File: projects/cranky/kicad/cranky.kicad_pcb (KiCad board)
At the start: 2 copper layers, 50 x 50 mm, 51 parts, among them CON1 USB-MINI-B, P1 ISP, P2 CONN_01X04, P3 CONN_01X04, P4 CONN_01X04, P5 CONN_01X04, Q1 2N7002P, Q2 2N7002P, Q3 ISL9V3040D3ST, Q4 ISL9V3040D3ST, Q5 VND5N07, Q6 VND5N07, SW1 SW_PUSH_SMALL, SW2 SW_PUSH_SMALL, U1 ATMEGA32U4-A, U2 LTV-826S, U3 LM7805CT, X1 16MHz

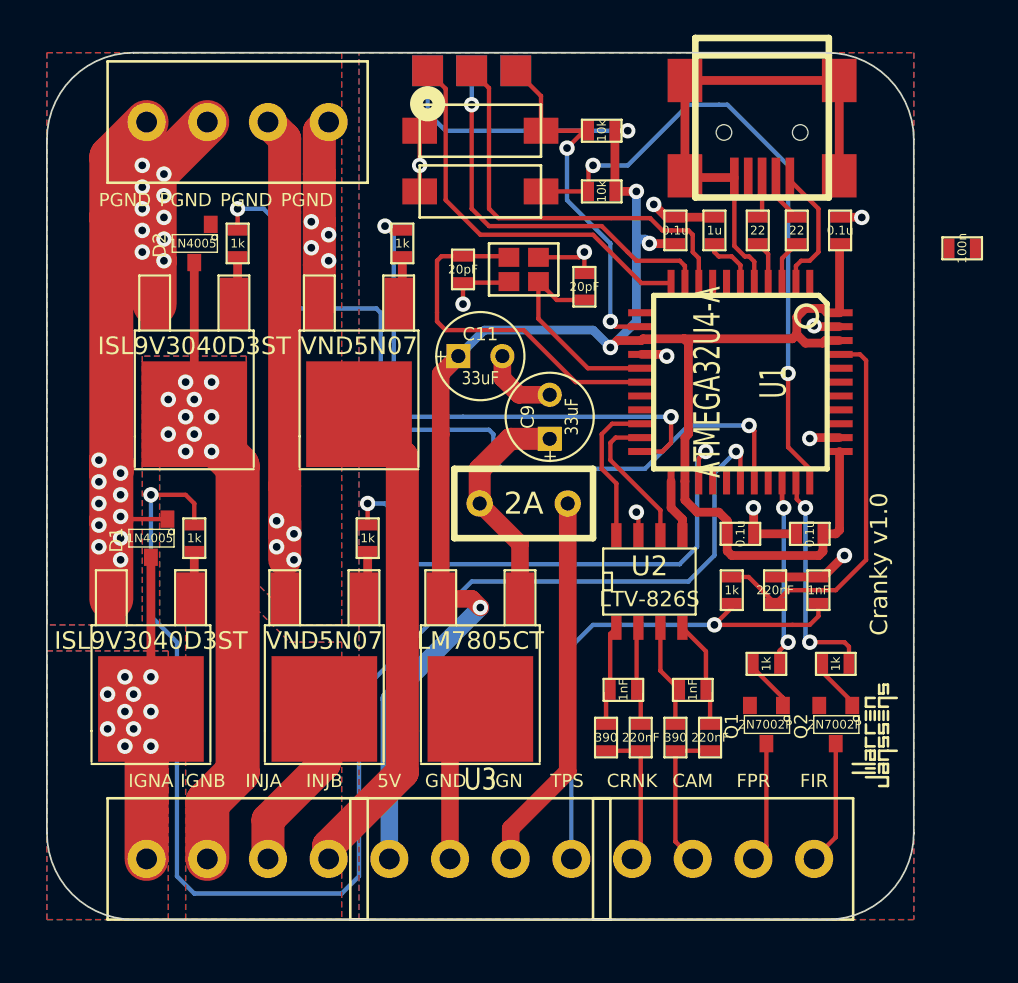
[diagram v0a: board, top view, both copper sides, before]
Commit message: routing new cranky board
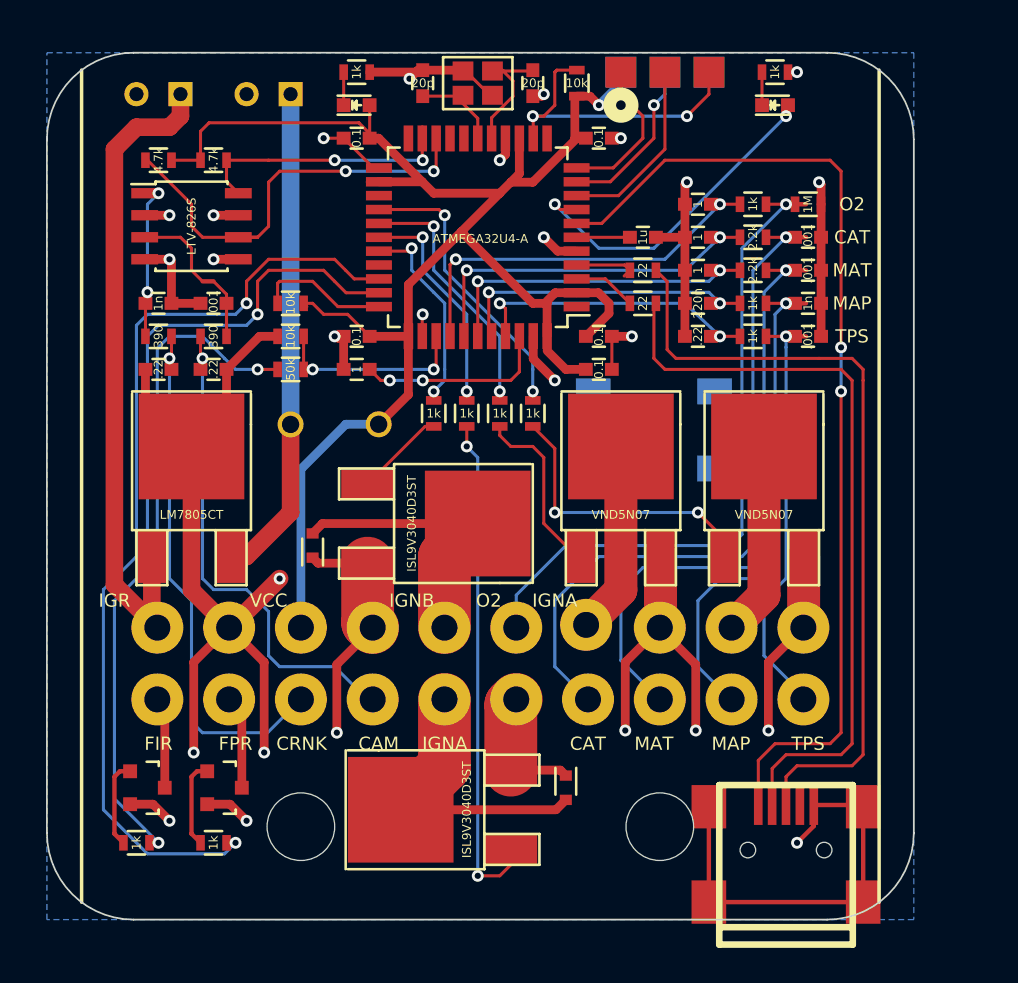
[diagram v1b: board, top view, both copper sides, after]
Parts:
- removed P3, P4, P5: CONN_01X04, SCREW_TERMINAL_4
- removed WJ10: VAL**, WJ10
- added C17: 0.1, Capacitors_SMD:C_0603, F.Cu at (76.8, 86.4)
- added C18: 1n, Capacitors_SMD:C_0603, F.Cu at (88.9, 84.5)
- added C19: .001, Capacitors_SMD:C_0603, F.Cu at (88.9, 80.6)
- added C20: .001, Capacitors_SMD:C_0603, F.Cu at (88.9, 82.5)
- added C21: 220n, Capacitors_SMD:C_0603, F.Cu at (82.5, 84.5)
- added C22: 1, Capacitors_SMD:C_0603, F.Cu at (82.5, 80.6)
- added C23: 1, Capacitors_SMD:C_0603, F.Cu at (82.5, 82.5)
- added C24: 1, Capacitors_SMD:C_0603, F.Cu at (82.5, 78.7)
- added D3: Led_Small, LEDs:LED-0603, F.Cu at (62.9, 73.0)
- added D4: Led_Small, LEDs:LED-0603, F.Cu at (87.0, 73.0)
- added R14: 4.7k, Resistors_SMD:R_0603, F.Cu at (54.6, 76.2)
- added R15: 4.7k, Resistors_SMD:R_0603, F.Cu at (51.4, 76.2)
- added R16: 1M, Resistors_SMD:R_0603, F.Cu at (88.9, 78.7)
- added R17: 50k, Resistors_SMD:R_0603, F.Cu at (59.1, 88.3)
- added R18: 1k, Resistors_SMD:R_0603, F.Cu at (85.7, 84.5)
- added R19: 2.2k, Resistors_SMD:R_0603, F.Cu at (85.7, 80.6)
- added R20: 2.2k, Resistors_SMD:R_0603, F.Cu at (85.7, 82.5)
- added R21: 1k, Resistors_SMD:R_0603, F.Cu at (85.7, 78.7)
- added R22: 10k, Resistors_SMD:R_0603, F.Cu at (59.1, 86.4)
- added R23: 1k, Resistors_SMD:R_0603, F.Cu at (62.9, 71.1)
- added R24: 1k, Resistors_SMD:R_0603, F.Cu at (87.0, 71.1)
- added WJ20: VAL**, DigitalCave:WJ20, B.Cu at (69.2, 81.3)
- C1, C2, C6: value 220nF -> .22; footprint SM0603_VALUE -> Capacitors_SMD:C_0603
- C10, C7: value 20pF -> 20p; footprint SM0603_VALUE -> Capacitors_SMD:C_0603
- C11, C9: value 33uF -> 33; footprint C1V5 -> Discret:C1V5H; moved to B.Cu
- C12, C13, C14, C15: value 0.1u -> 0.1; footprint SM0603_VALUE -> Capacitors_SMD:C_0603
- C16: value 100n -> 1; footprint custom:SM0603_VALUE -> Capacitors_SMD:C_0603
- C3, C5: value 1nF -> .001; footprint SM0603_VALUE -> Capacitors_SMD:C_0603
- C4: value 1nF -> 1n; footprint SM0603_VALUE -> Capacitors_SMD:C_0603
- C8: footprint SM0603_VALUE -> Capacitors_SMD:C_0603
- CON1: footprint USB_MINI_B_fixed -> DigitalCave:USB_MINI_B_fixed
- D1, D2: footprint SOT23 -> Diodes_SMD:SOD-523
- F1: footprint FUSE_TE5 -> Fuse_Holders_and_Fuses:Fuse_TE5_Littlefuse-395Series; moved to B.Cu
- P1: footprint ISP_EDGE -> DigitalCave:ISP_EDGE
- P2: value CONN_01X04 -> AMP794106; footprint SCREW_TERMINAL_4 -> DigitalCave:AMP794106; moved to B.Cu
- Q1, Q2: footprint SOT23 -> TO_SOT_Packages_SMD:SOT-23
- Q3, Q4, Q5, Q6, U3: footprint DPAK2 -> TO_SOT_Packages_SMD:TO-252-2Lead
- R1, R10, R11, R12, R13, R2, R3, R4, R5, R6, R7, R8, R9: footprint SM0603_VALUE -> Resistors_SMD:R_0603
- SW1, SW2: footprint SW_6x3 -> DigitalCave:SW_6x3; moved to B.Cu
- U1: footprint TQFP44 -> Housings_QFP:TQFP-44_10x10mm_Pitch0.8mm
- U2: footprint SO8E -> Housings_SOIC:SOIC-8_3.9x4.9mm_Pitch1.27mm
- X1: footprint crystal_smd_2.5x2 -> DigitalCave:CRYSTAL_SMD_2.5x2
- moved CON1 43.1 mm to (87.6, 116.8), turned to 90 degrees
- moved R8 41.6 mm to (50.2, 115.6)
- moved Q2 39.9 mm to (50.8, 112.4), turned to 270 degrees
- moved P2 36.1 mm to (70.0, 107.3), turned to 180 degrees
- moved C2 35.7 mm to (54.6, 88.3), turned to 0 degrees
- moved C16 35.6 mm to (62.9, 88.3), turned to 180 degrees
- moved C5 35.5 mm to (54.6, 84.5), turned to 180 degrees
- moved R2 35.3 mm to (54.6, 86.4), turned to 180 degrees
- moved C1 35.0 mm to (51.4, 88.3), turned to 180 degrees
- moved C4 34.9 mm to (51.4, 84.5)
- moved R1 34.7 mm to (51.4, 86.4), turned to 0 degrees
- moved R7 33.5 mm to (54.6, 115.6)
- moved U2 33.4 mm to (53.3, 80.0)
- moved Q1 31.5 mm to (55.2, 112.4), turned to 270 degrees
- moved C9 29.2 mm to (51.4, 72.4), turned to 180 degrees
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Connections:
- net /X1 renamed /X+
- net /X2 renamed /X-
- C11 pad 1: VCC -> Net-(C11-Pad1)
- C13 pad 1: VCC -> DGND
- C13 pad 2: DGND -> VCC
- C15 pad 1: VCC -> DGND
- C15 pad 2: DGND -> VCC
- C16 pad 1: DGND -> Net-(C16-Pad1)
- C16 pad 2: Net-(C16-Pad2) -> DGND
- C8 pad 1: DGND -> /UCAP
- C8 pad 2: /UCAP -> DGND
- C9 pad 1: Net-(C9-Pad1) -> /IGR
- CON1 pad 1: Net-(CON1-Pad1) -> /VBUS
- CON1 pad 2: Net-(CON1-Pad2) -> /UDM
- CON1 pad 3: Net-(CON1-Pad3) -> /UDP
- CON1 pad 4: Net-(CON1-Pad4) -> (no net)
- CON1 pad 5: Net-(CON1-Pad5) -> DGND
- CON1 pad 6: Net-(CON1-Pad6) -> DGND
- CON1 pad 7: Net-(CON1-Pad7) -> DGND
- CON1 pad 8: Net-(CON1-Pad8) -> DGND
- CON1 pad 9: Net-(CON1-Pad9) -> DGND
- D1 pad 1: GNDPWR -> DGND
- D2 pad 1: GNDPWR -> DGND
- F1 pad 1: Net-(C9-Pad1) -> Net-(C11-Pad1)
- F1 pad 2: /IGR -> VCC
- P2 pad 1: GNDPWR -> /IGR
- P2 pad 2: GNDPWR -> DGND
- P2 pad 3: GNDPWR -> VCC
- P2 pad 4: GNDPWR -> DGND
- Q3 pad 3: GNDPWR -> DGND
- Q4 pad 3: GNDPWR -> DGND
- Q5 pad S: GNDPWR -> DGND
- Q6 pad S: GNDPWR -> DGND
- R12 pad 2: /PD4 -> /PD7
- R13 pad 2: /PD5 -> /PD6
- U1 pad 1: Net-(U1-Pad1) -> (no net)
- U1 pad 12: Net-(U1-Pad12) -> (no net)
- U1 pad 18: Net-(U1-Pad18) -> (no net)
- U1 pad 19: Net-(U1-Pad19) -> (no net)
- U1 pad 2: /UVCC -> VCC
- U1 pad 22: /PD5 -> (no net)
- U1 pad 25: /PD4 -> (no net)
- U1 pad 26: Net-(U1-Pad26) -> /PD6
- U1 pad 27: Net-(U1-Pad27) -> /PD7
- U1 pad 30: Net-(U1-Pad30) -> (no net)
- U1 pad 36: Net-(U1-Pad36) -> /ADC7
- U1 pad 37: Net-(U1-Pad37) -> /ADC6
- U1 pad 38: Net-(U1-Pad38) -> /ADC5
- U1 pad 39: Net-(U1-Pad39) -> /ADC4
- U1 pad 40: Net-(U1-Pad40) -> /ADC1
- U1 pad 42: Net-(C16-Pad2) -> Net-(C16-Pad1)
- U1 pad 5: /UGND -> DGND
- U2 pad 6: /INT3 -> /INT2
- U2 pad 8: /INT2 -> /INT3
- U3 pad 1: Net-(C9-Pad1) -> /IGR
- U3 pad 3: VCC -> Net-(C11-Pad1)
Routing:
- net GNDPWR: track 125.8 -> 0.00 mm, vias 28 -> 0
- net DGND: track 60.2 -> 184.2 mm, vias 11 -> 27
- net /PB4: track 80.5 -> 13.0 mm
- net /VBUS: track 0.00 -> 57.4 mm, vias 0 -> 2
- net /UDM: track 0.00 -> 43.4 mm
- net /UDP: track 2.39 -> 45.4 mm
- net /PC6: track 12.3 -> 55.0 mm
- net /IGR: track 21.9 -> 62.4 mm, vias 0 -> 1
- net /CAT: track 0.00 -> 40.0 mm, vias 0 -> 1
- net /O2: track 0.00 -> 38.7 mm, vias 0 -> 1
- net /PB5: track 48.5 -> 11.8 mm
- net /MAT: track 0.00 -> 35.5 mm, vias 0 -> 1
- net /IGNB: track 52.0 -> 16.6 mm, vias 10 -> 0
- net /PC7: track 13.0 -> 48.2 mm
- net /PD5: track 31.4 -> 0.00 mm, vias 2 -> 0
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- removed copper zone on B.Cu, net /IGNA
- removed copper zone on F.Cu, net /IGNA
- removed copper zone on B.Cu, net /IGNB
- removed copper zone on F.Cu, net /IGNB
- removed copper zone on F.Cu, net DGND
- removed copper zone on B.Cu, net GNDPWR
- removed copper zone on F.Cu, net GNDPWR
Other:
- net class Default: clearance 0.2032 -> 0.1778; trace_width 0.254 -> 0.1778; via_dia 0.889 -> 0.6858; via_drill 0.635 -> 0.3556
- rule trace_clearance: 0.2032 -> 0.1778
- rule trace_min: 0.254 -> 0.1778
- rule via_min_drill: 0.508 -> 0.3556
- rule via_min_size: 0.889 -> 0.6858
- board text added: "+"
- board text added: "CAT"
- board text added: "Cranky ECM 1.0"
- board text added: "IGR"
- board text added: "MAP"
- board text added: "MAT"
- board text added: "O2"
- board text added: "VCC"
- board text removed: "5V"
- board text removed: "Cranky v1.0"
- board text removed: "GND"
- board text removed: "IGN"
- board text removed: "INJA"
- board text removed: "INJB"
- board text removed: "PGND"
